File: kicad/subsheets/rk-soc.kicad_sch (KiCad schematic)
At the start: 22 parts, among them U5 RK3566

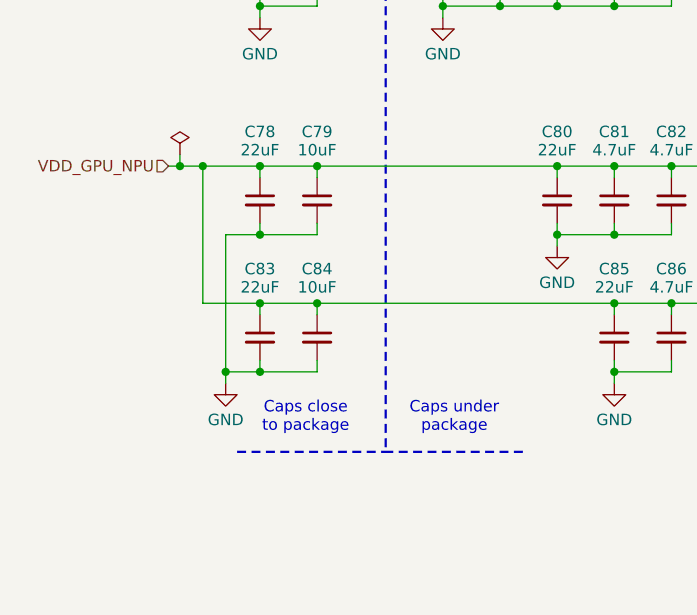
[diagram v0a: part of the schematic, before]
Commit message: Minor tweaks + annotations
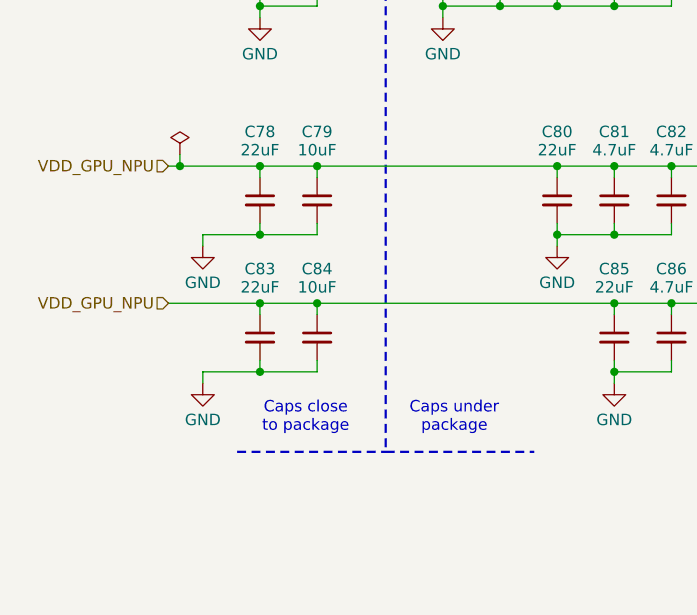
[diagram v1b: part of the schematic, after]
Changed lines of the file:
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@@
 	)
 	(junction
-		(at 69.85 120.65)
-		(diameter 0)
-		(color 0 0 0 0)
-	)
-	(junction
 		(at 106.68 41.91)
 		(diameter 0)
@@
 	)
 	(junction
-		(at 67.31 97.79)
-		(diameter 0)
-		(color 0 0 0 0)
-	)
-	(junction
 		(at 113.03 105.41)
 		(diameter 0)
@@
 	(wire
 		(pts
-			(xy 69.85 121.92) (xy 69.85 120.65)
+			(xy 67.31 121.92) (xy 67.31 120.65)
 		)
 		(stroke
@@
 	(wire
 		(pts
-			(xy 69.85 105.41) (xy 69.85 120.65)
-		)
-		(stroke
-			(width 0)
-			(type default)
-		)
-	)
-	(wire
-		(pts
 			(xy 171.45 72.39) (xy 167.64 72.39)
 		)
@@
 	(wire
 		(pts
-			(xy 69.85 105.41) (xy 73.66 105.41)
+			(xy 67.31 105.41) (xy 73.66 105.41)
 		)
 		(stroke
@@
 		)
 	)
+	(polyline
+		(pts
+			(xy 87.63 129.54) (xy 104.14 129.54)
+		)
+		(stroke
+			(width 0.25)
+			(type dash)
+			(color 0 0 255 1)
+		)
+	)
 	(wire
 		(pts
@@
 	(wire
 		(pts
-			(xy 73.66 120.65) (xy 69.85 120.65)
+			(xy 73.66 120.65) (xy 67.31 120.65)
 		)
 		(stroke
@@
 	(wire
 		(pts
+			(xy 63.5 113.03) (xy 73.66 113.03)
+		)
+		(stroke
+			(width 0)
+			(type default)
+		)
+	)
+	(wire
+		(pts
 			(xy 167.64 52.07) (xy 196.85 52.07)
 		)
@@
 	(wire
 		(pts
-			(xy 67.31 97.79) (xy 64.77 97.79)
+			(xy 64.77 97.79) (xy 73.66 97.79)
 		)
 		(stroke
@@
 	(wire
 		(pts
-			(xy 67.31 97.79) (xy 67.31 113.03)
-		)
-		(stroke
-			(width 0)
-			(type default)
-		)
-	)
-	(wire
-		(pts
 			(xy 113.03 80.01) (xy 113.03 78.74)
 		)
@@
 		)
 	)
-	(polyline
-		(pts
-			(xy 102.87 129.54) (xy 87.63 129.54)
-		)
-		(stroke
-			(width 0.25)
-			(type dash)
-			(color 0 0 255 1)
-		)
-	)
 	(wire
 		(pts
@@
 	(wire
 		(pts
-			(xy 67.31 97.79) (xy 73.66 97.79)
-		)
-		(stroke
-			(width 0)
-			(type default)
-		)
-	)
-	(wire
-		(pts
 			(xy 124.46 41.91) (xy 127 41.91)
 		)
@@
 	(wire
 		(pts
+			(xy 67.31 105.41) (xy 67.31 106.68)
+		)
+		(stroke
+			(width 0)
+			(type default)
+		)
+	)
+	(wire
+		(pts
 			(xy 73.66 113.03) (xy 80.01 113.03)
 		)
@@
 	(wire
 		(pts
-			(xy 67.31 113.03) (xy 73.66 113.03)
-		)
-		(stroke
-			(width 0)
-			(type default)
-		)
-	)
-	(wire
-		(pts
 			(xy 73.66 120.65) (xy 73.66 119.38)
 		)
@@
 		)
 	)
+	(hierarchical_label "VDD_GPU_NPU"
+		(shape input)
+		(at 63.5 113.03 180)
+		(effects
+			(font
+				(size 1.27 1.27)
+			)
+			(justify right)
+		)
+	)
 	(hierarchical_label "VCCA_1V8"
 		(shape input)
@@
 	(symbol
 		(lib_id "power:GND")
-		(at 69.85 121.92 0)
+		(at 67.31 121.92 0)
 		(mirror y)
 		(unit 1)
@@
 		(fields_autoplaced yes)
 		(property "Reference" "#PWR063"
-			(at 69.85 128.27 0)
+			(at 67.31 128.27 0)
 			(effects
 				(font
@@
 		)
 		(property "Value" "GND"
-			(at 69.85 125.984 0)
+			(at 67.31 125.984 0)
 			(effects
 				(font
@@
 		)
 		(property "Footprint" ""
-			(at 69.85 121.92 0)
+			(at 67.31 121.92 0)
 			(effects
 				(font
@@
 		)
 		(property "Datasheet" ""
-			(at 69.85 121.92 0)
+			(at 67.31 121.92 0)
 			(effects
 				(font
@@
 		)
 		(property "Description" "Power symbol creates a global label with name \"GND\" , ground"
-			(at 69.85 121.92 0)
+			(at 67.31 121.92 0)
 			(effects
 				(font
@@
 					(unit 1)
 				)
+			)
+		)
+	)
+	(symbol
+		(lib_id "power:GND")
+		(at 67.31 106.68 0)
+		(mirror y)
+		(unit 1)
+		(exclude_from_sim no)
+		(in_bom yes)
+		(on_board yes)
+		(dnp no)
+		(fields_autoplaced yes)
+		(property "Reference" "#PWR0108"
+			(at 67.31 113.03 0)
+			(effects
+				(font
+					(size 1.27 1.27)
+				)
+				(hide yes)
+			)
+		)
+		(property "Value" "GND"
+			(at 67.31 110.744 0)
+			(effects
+				(font
+					(size 1.27 1.27)
+				)
+			)
+		)
+		(property "Footprint" ""
+			(at 67.31 106.68 0)
+			(effects
+				(font
+					(size 1.27 1.27)
+				)
+				(hide yes)
+			)
+		)
+		(property "Datasheet" ""
+			(at 67.31 106.68 0)
+			(effects
+				(font
+					(size 1.27 1.27)
+				)
+				(hide yes)
+			)
+		)
+		(property "Description" "Power symbol creates a global label with name \"GND\" , ground"
+			(at 67.31 106.68 0)
+			(effects
+				(font
+					(size 1.27 1.27)
+				)
+				(hide yes)
+			)
+		)
+		(pin "1"
+		)
+		(instances
+			(project "srad-camera"
+				(path "/da62c771-e8c9-451f-8df1-ec995aadcb11/279fc251-45a8-41a3-8fcf-5855d7fe07da"
+					(reference "#PWR0108")
+					(unit 1)
+				)
